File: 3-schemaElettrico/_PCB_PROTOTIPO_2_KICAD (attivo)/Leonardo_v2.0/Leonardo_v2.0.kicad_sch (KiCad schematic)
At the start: 27 parts, among them J1 Screw_Terminal_01x02, J2 Conn_01x06_Pin, J3 Conn_01x06_Pin, J4 Conn_01x04_Pin, J5 Conn_01x04_Pin, J6 Conn_01x04_Pin, J7 Conn_01x04_Pin, Q1 BC817, Q2 BC807, U2 DC_DC_small, U3 DC_DC_small

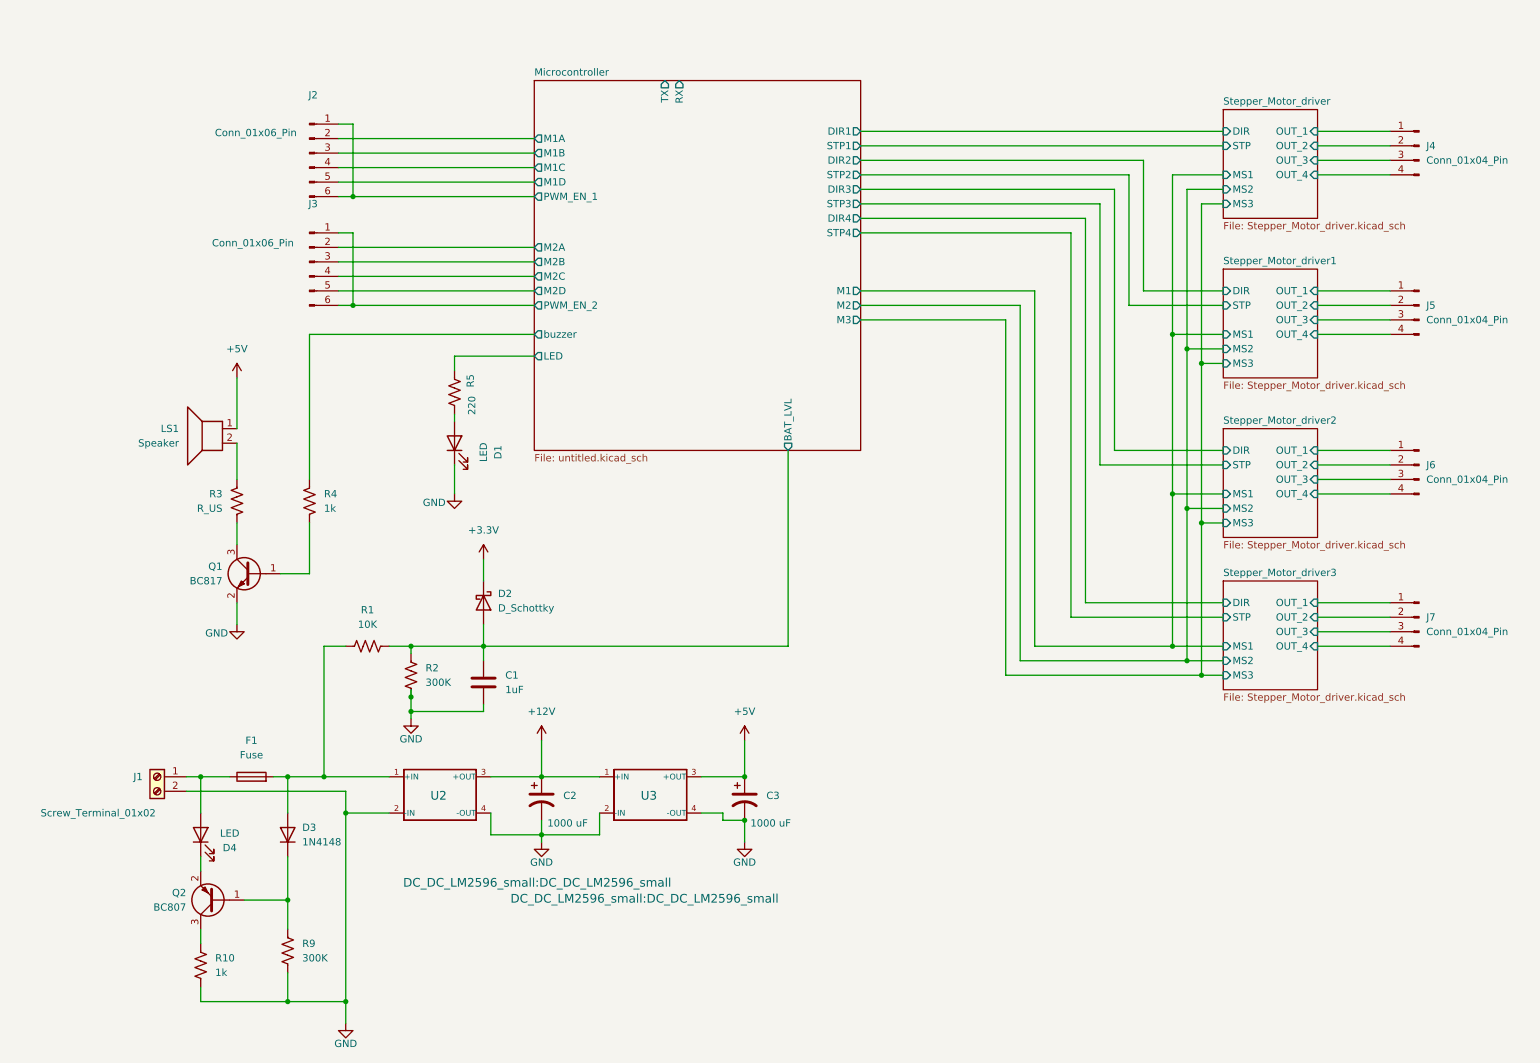
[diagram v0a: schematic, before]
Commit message: OK
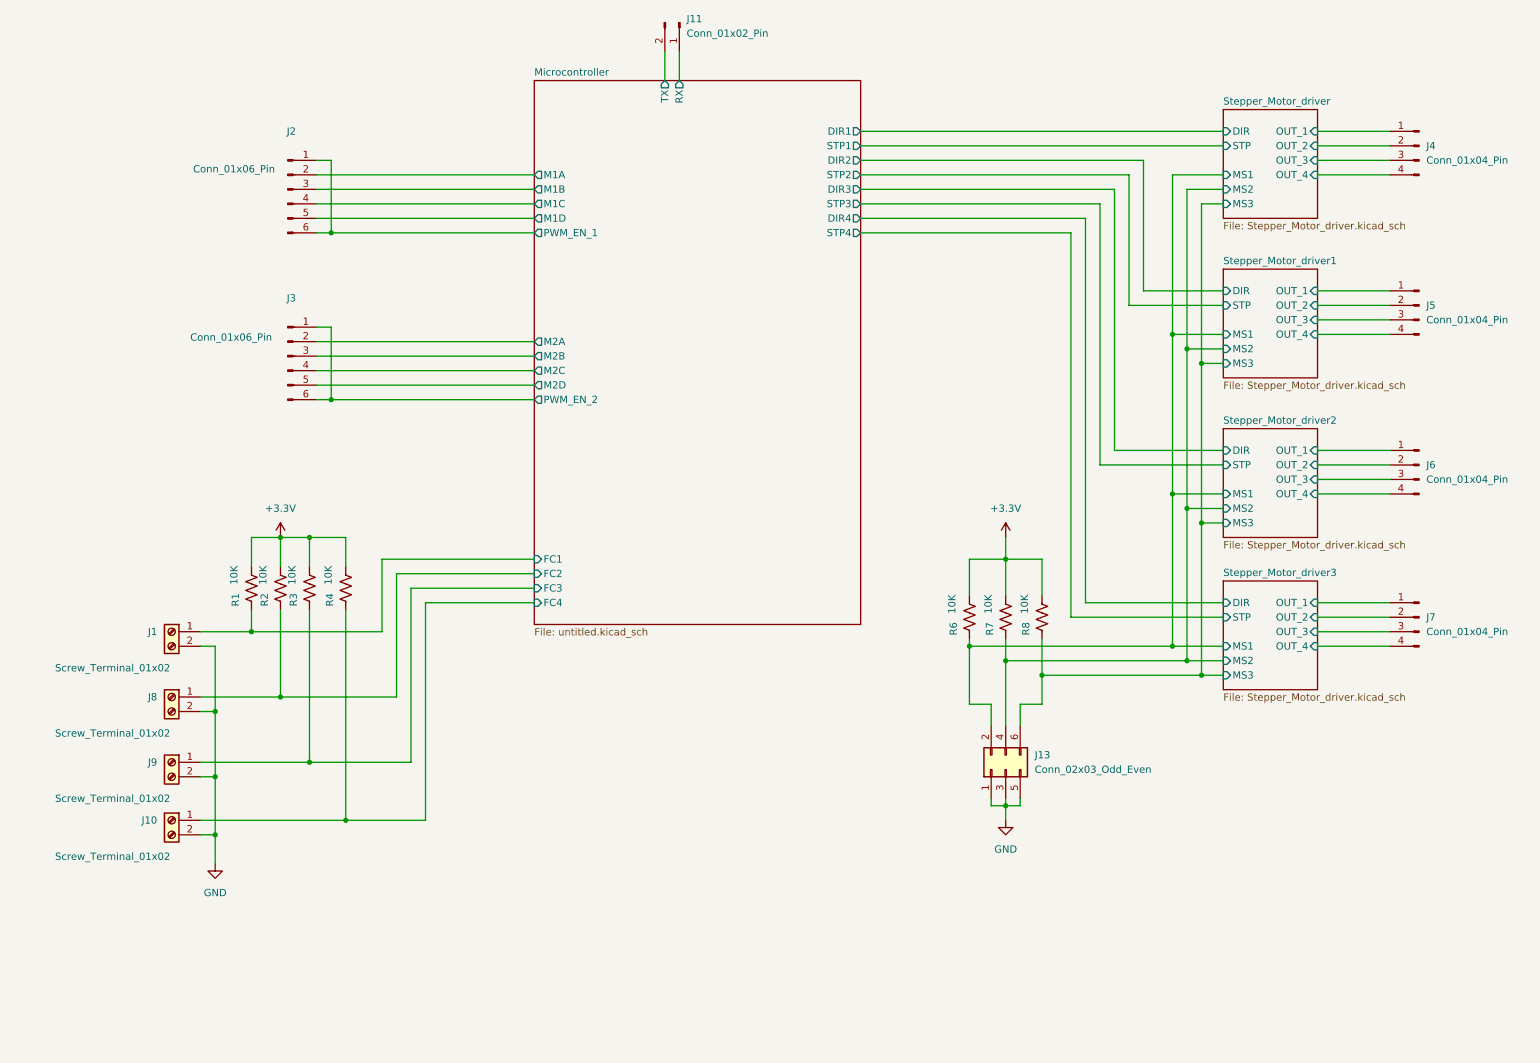
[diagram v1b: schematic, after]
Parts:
- removed C1: 1uF, Capacitor_SMD:C_0805_2012Metric_Pad1.18x1.45mm_HandSolder, symbol Device:C
- removed C2, C3: 1000 uF, Capacitor_THT:CP_Radial_D10.0mm_P5.00mm, symbol Device:C_Polarized_US
- removed D1, D4: LED, LED_THT:LED_D3.0mm_FlatTop, symbol Device:LED
- removed D2: D_Schottky, Diode_THT:D_5KPW_P12.70mm_Horizontal, symbol Device:D_Schottky
- removed D3: 1N4148, Diode_THT:D_DO-35_SOD27_P7.62mm_Horizontal, symbol Diode:1N4148
- removed F1: Fuse, Fuse:Fuse_1812_4532Metric_Pad1.30x3.40mm_HandSolder, symbol Device:Fuse
- removed LS1: Speaker, Buzzer_Beeper:Buzzer_TDK_PS1240P02BT_D12.2mm_H6.5mm, symbol Device:Speaker
- removed Q1: BC817, Package_TO_SOT_SMD:SOT-23-3, symbol Transistor_BJT:BC817
- removed Q2: BC807, Package_TO_SOT_SMD:SOT-23, symbol Transistor_BJT:BC807
- removed R10: 1k, Resistor_SMD:R_0805_2012Metric, symbol Device:R_US
- removed R5: 220, Resistor_SMD:R_0805_2012Metric, symbol Device:R_US
- removed R9: 300K, Resistor_SMD:R_0805_2012Metric, symbol Device:R_US
- removed U2, U3: DC_DC_small, DC_DC_LM2596_small:DC_DC_LM2596_small, symbol Custom_dc_dc_small:DC_DC_small
- added J10, J8, J9: Screw_Terminal_01x02, TerminalBlock_Phoenix:TerminalBlock_Phoenix_MKDS-1,5-2_1x02_P5.00mm_Horizontal, symbol Connector:Screw_Terminal_01x02
- added J11: Conn_01x02_Pin, symbol Connector:Conn_01x02_Pin
- added J13: Conn_02x03_Odd_Even, Connector_PinHeader_2.54mm:PinHeader_2x03_P2.54mm_Vertical, symbol Connector_Generic:Conn_02x03_Odd_Even
- added R6, R7, R8: 10K, Resistor_SMD:R_0805_2012Metric, symbol Device:R_US
- R2: value 300K -> 10K
- R3: value R_US -> 10K
- R4: value 1k -> 10K
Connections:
- net +3.3V: now also R1.2, R2.2, R3.2, R4.2, R6.2, R7.2, R8.2
- net GND: now also J10.2 (Pin_2), J13.1 (Pin_1), J13.3 (Pin_3), J13.5 (Pin_5), J8.2 (Pin_2), J9.2 (Pin_2); no longer R2.2
- net Microcontroller/RX: now also J11.1 (Pin_1)
- net Microcontroller/TX: now also J11.2 (Pin_2)
- net Microcontroller/FC1: now reaches R1.1
- net Microcontroller/FC1: now also J1.1 (Pin_1)
- net Microcontroller/FC3: now reaches R3.1
- net Microcontroller/FC3: now also J9.1 (Pin_1)
- net Microcontroller/BAT_LVL renamed Microcontroller/FC2
- net Microcontroller/FC2: now also J8.1 (Pin_1); no longer R1.2
- net Microcontroller/buzzer renamed Microcontroller/FC4
- net Microcontroller/FC4: now also J10.1 (Pin_1)
- new net Stepper_Motor_driver/MS1: J13.2 (Pin_2), R6.1
- new net Stepper_Motor_driver/MS2: J13.4 (Pin_4), R7.1
- new net Stepper_Motor_driver/MS3: J13.6 (Pin_6), R8.1
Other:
- sheet Microcontroller ports: added FC1, FC2, FC3, FC4; removed BAT_LVL, LED, M1, M2, M3, buzzer
- moved on the sheet: J1, J2, J3
